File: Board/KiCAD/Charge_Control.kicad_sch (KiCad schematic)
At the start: 53 parts, among them Q1 AON7408, Q10 AON7407, Q2 AON7408, Q3 AON7408, Q4 AON7408, U1 BQ25730RSNR, U3 LTC2943CDD#PBF

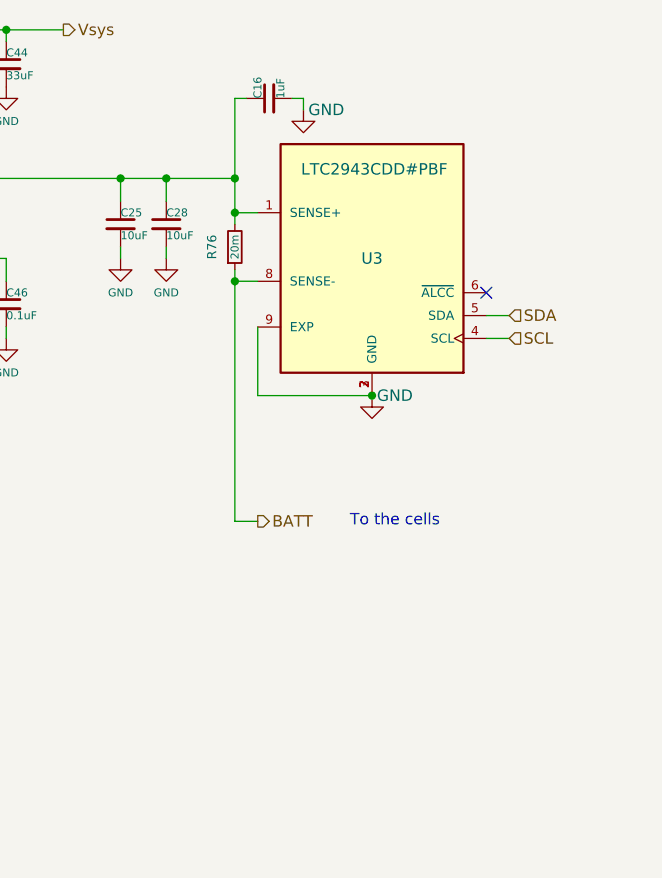
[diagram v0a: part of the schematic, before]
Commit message: finished PCB
PCB completed @andrewgreenberg
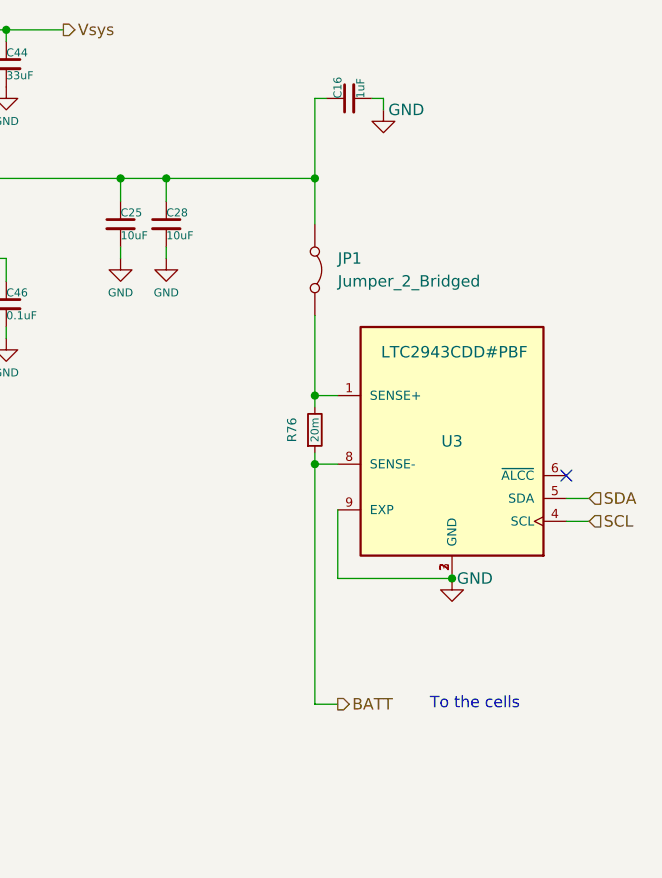
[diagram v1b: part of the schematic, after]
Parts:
- added JP1: Jumper_2_Bridged, TestPoint:TestPoint_2Pads_Pitch2.54mm_Drill0.8mm, symbol Jumper:Jumper_2_Bridged
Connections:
- net at C16.1, C23.2, C25.1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: now also JP1.1 (A); no longer R76.2, U3.1 (SENSE+)
- new net: JP1.2 (B), R76.2, U3.1 (SENSE+)
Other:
- moved on the sheet: C16, R76, U3
